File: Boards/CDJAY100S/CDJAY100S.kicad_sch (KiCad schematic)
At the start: 50 parts, among them SW1 RotaryEncoder_Switch, U1 HT1632C-52LQFP

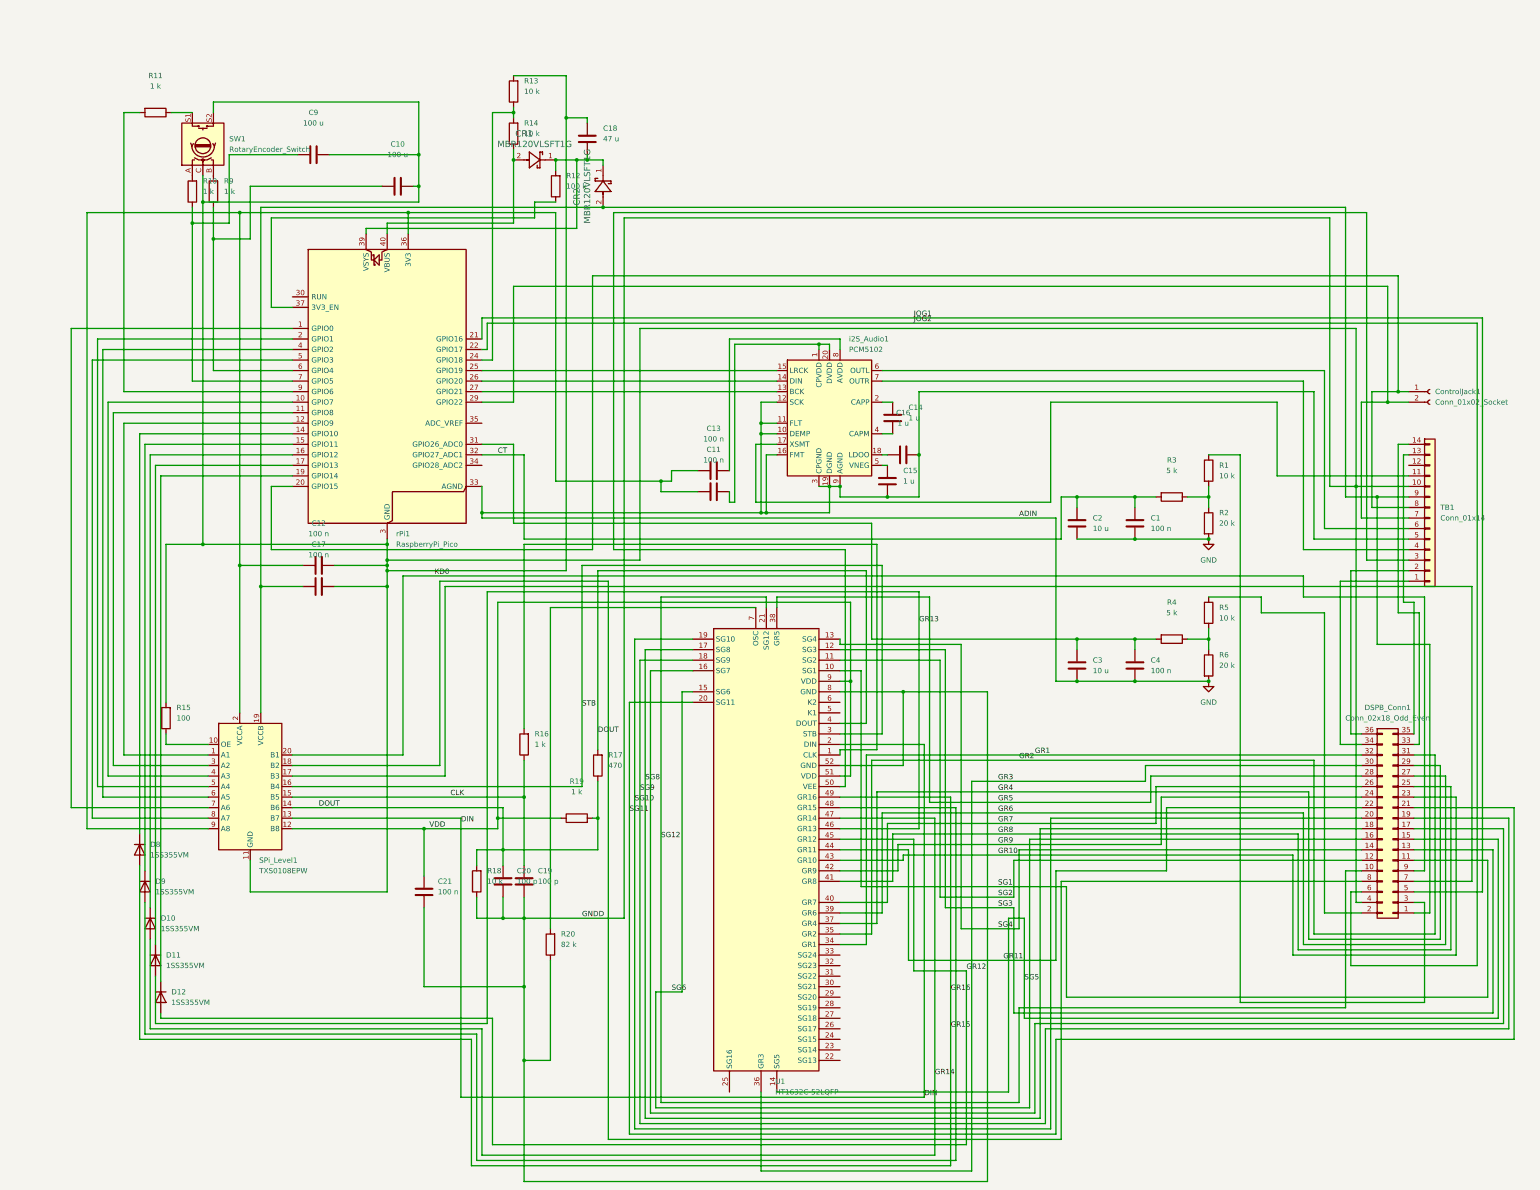
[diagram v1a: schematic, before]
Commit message: Revision 1.1 of the PCB and Schematics.
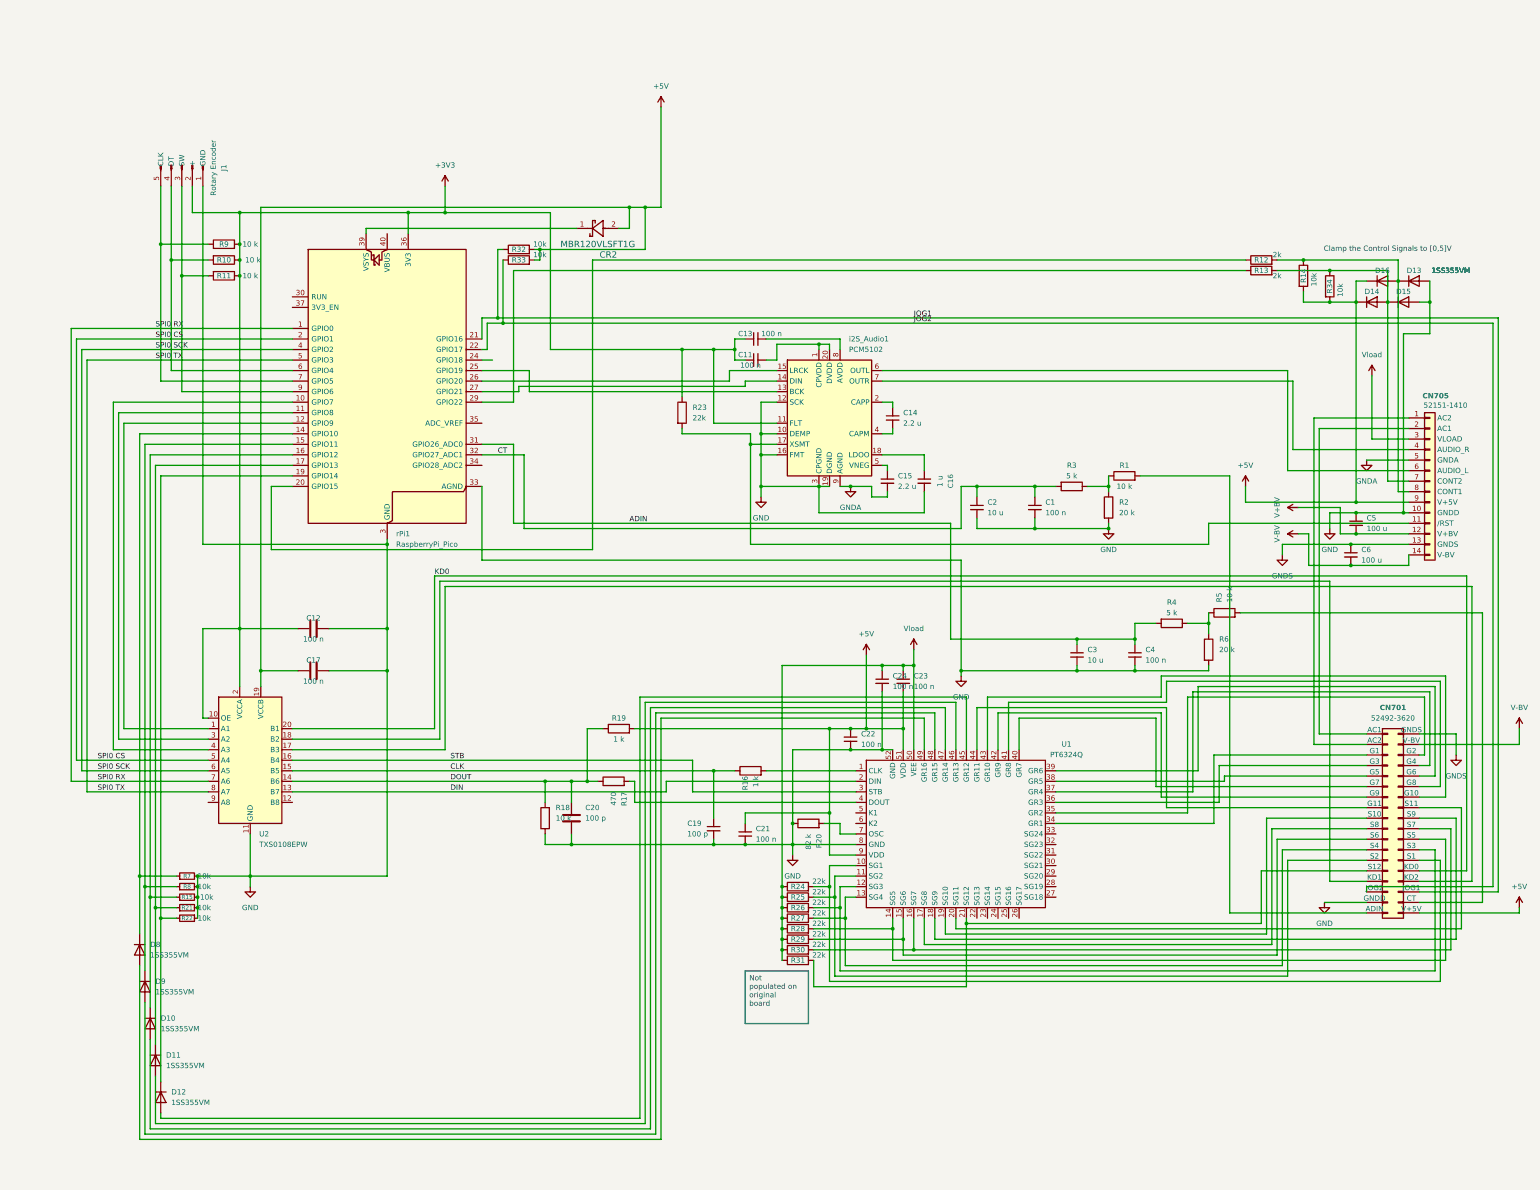
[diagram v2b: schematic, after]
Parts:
- removed C10, C9: 100 u, Capacitor_SMD:C_1206_3216Metric_Pad1.33x1.80mm_HandSolder, symbol Device:C
- removed C18: 47 u, Capacitor_SMD:C_1206_3216Metric_Pad1.33x1.80mm_HandSolder, symbol Device:C
- removed C19: 100 p, Capacitor_SMD:C_1206_3216Metric_Pad1.33x1.80mm_HandSolder, symbol Device:C
- removed C21: 100 n, Capacitor_SMD:C_1206_3216Metric_Pad1.33x1.80mm_HandSolder, symbol Device:C
- removed CR1: MBR120VLSFT1G, SDO_SOD-123FL_ONS, symbol 2026-07-07_11-12-20:MBR120VLSFT1G
- removed ControlJack1: Conn_01x02_Socket, Connector_Hirose:Hirose_DF13-02P-1.25DSA_1x02_P1.25mm_Vertical, symbol Connector:Conn_01x02_Socket
- removed DSPB_Conn1: Conn_02x18_Odd_Even, 52045-3645:ConnectorFPC&FFC_MOL52045-3645-36P, symbol Connector_Generic:Conn_02x18_Odd_Even
- removed R15: 100, Resistor_SMD:R_1206_3216Metric_Pad1.30x1.75mm_HandSolder, symbol Device:R
- removed SW1: RotaryEncoder_Switch, Connector_PinHeader_2.54mm:PinHeader_1x05_P2.54mm_Vertical, symbol Device:RotaryEncoder_Switch
- removed TB1: Conn_01x14, Connector_PinHeader_2.00mm:PinHeader_1x14_P2.00mm_Vertical, symbol Connector_Generic:Conn_01x14
- added C19: 100 p, Capacitor_SMD:C_1206_3216Metric_Pad1.33x1.80mm_HandSolder, symbol Device:C_Small
- added C21, C22, C23, C24: 100 n, Capacitor_SMD:C_1206_3216Metric_Pad1.33x1.80mm_HandSolder, symbol Device:C_Small
- added C5, C6: 100 u, Capacitor_SMD:C_1206_3216Metric_Pad1.33x1.80mm_HandSolder, symbol Device:C_Small
- added CN701: 52492-3620, 52045-3645:ConnectorFPC&FFC_MOL52045-3645-36P_1, symbol Connector_Generic:Conn_02x18_Odd_Even
- added CN705: 52151-1410, Connector_PinHeader_2.00mm:PinHeader_1x14_P2.00mm_Vertical, symbol Connector_Generic:Conn_01x14
- added D13, D14, D15, D16: 1SS355VM, Diode_SMD:Nexperia_CFP3_SOD-123W, symbol Diode:1SS355VM
- added J1: Rotary Encoder, Connector_PinHeader_2.54mm:PinHeader_1x05_P2.54mm_Vertical, symbol Connector:Conn_01x05_Pin
- added R15, R21, R22, R7, R8: 10k, Resistor_SMD:R_1206_3216Metric_Pad1.30x1.75mm_HandSolder, symbol Device:R_Small
- added R23, R24, R25, R26, R27, R28, R29, R30, R31: 22k, Resistor_SMD:R_1206_3216Metric_Pad1.30x1.75mm_HandSolder, symbol Device:R
- added R32, R33, R34: 10k, Resistor_SMD:R_1206_3216Metric_Pad1.30x1.75mm_HandSolder, symbol Device:R
- C1, C11, C13, C16, C2, C3, C4: symbol Device:C -> Device:C_Small
- C14, C15: value 1 u -> 2.2 u; symbol Device:C -> Device:C_Small
- CR2: footprint SDO_SOD-123FL_ONS -> Diode_SMD:Nexperia_CFP3_SOD-123W
- D10, D11, D12, D8, D9: footprint Diode_SMD:D_SOD-323F -> Diode_SMD:Nexperia_CFP3_SOD-123W
- R10, R11, R9: value 1 k -> 10 k
- R12: value 100 k -> 2k
- R13: value 10 k -> 2k
- R14: value 10 k -> 10k
- U1: value HT1632C-52LQFP -> PT6324Q; footprint Package_QFP:LQFP-52_14x14mm_P1mm -> Package_QFP:QFP-52_14x14mm_P1mm_1; symbol Driver_LED:HT1632C-52LQFP -> CDjay:PT6324
- renumbered SPi_Level1 to U2
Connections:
- net CLK: now also C19.1
- net DOUT: now also R19.1; no longer R17.2, R19.2, U1.4 (DOUT)
- net GND: now also C12.2, C17.2, C20.2, R18.1, R20.1, U1.52 (GND), U1.8 (GND), U2.11 (GND), rPi1.13 (GND), rPi1.18 (GND), rPi1.23 (GND), rPi1.28 (GND), rPi1.3 (GND), rPi1.38 (GND), rPi1.8 (GND), C19.2, C21.2, C22.2, C24.2, C5.1, CN701.4 (GNDD), CN705.10 (GNDD), D13.2 (A), D15.2 (A), J1.1 (GND), R15.2, R21.2, R22.1, R7.2, R8.2; no longer C15.2, i2S_Audio1.11 (FLT), i2S_Audio1.9 (AGND)
- net JOG1: now also CN701.5 (JOG1), R32.1
- net JOG2: now also CN701.6 (JOG2), R33.1
- net KD0: now also CN701.9 (KD0)
- net at R5.1: now also R4.1, R6.1
- net at D9.1 (K), rPi1.15 (GPIO11): now also R8.1
- net at R10.2: now also rPi1.6 (GPIO4), J1.4 (DT)
- net +3V3: now reaches R9.2
- net +3V3: now also C11.1, C12.1, C13.1, R10.1, R11.1, U2.10 (OE), U2.2 (VCCA), i2S_Audio1.11 (FLT), rPi1.36 (3V3), J1.2 (+), R23.1
- net at U2.17 (B3): now also CN701.7 (KD2)
- net at U2.18 (B2): now also CN701.8 (KD1)
- net +5V: now reaches C17.1, CR2.2, U2.19 (VCCB)
- net +5V: now also R14.2, R19.2, U1.51 (VDD), U1.9 (VDD), C21.1, C22.1, C23.2, CN701.1 (V+5V), CN705.9 (V+5V), D14.1 (K), D16.1 (K), R32.2, R33.2, R34.2
- net SPI0 CS: now reaches U2.5 (A4), rPi1.2 (GPIO1)
- net SPI0 SCK: now reaches U2.6 (A5), rPi1.4 (GPIO2)
- net SPI0 RX: now reaches U2.7 (A6), rPi1.1 (GPIO0)
- net SPI0 TX: now reaches U2.8 (A7), rPi1.5 (GPIO3)
- net at rPi1.7 (GPIO5): now also R9.1, J1.5 (CLK); no longer R10.1
- net at D11.1 (K), rPi1.17 (GPIO13): now also R21.1
- net at i2S_Audio1.17 (XSMT): now also CN705.11 (/RST), R23.2
- net Vload: now reaches U1.50 (VEE)
- net Vload: now also C23.1, C24.1, CN705.3 (VLOAD), R24.1, R25.1, R26.1, R27.1, R28.1, R29.1, R30.1, R31.1
- net at i2S_Audio1.7 (OUTR): now also CN705.4 (AUDIO_R)
- net at i2S_Audio1.6 (OUTL): now also CN705.6 (AUDIO_L)
- net at rPi1.29 (GPIO22): now also R13.1
- net at rPi1.20 (GPIO15): now also R12.1
- net ADIN: now reaches C3.1, C4.1, R4.2, rPi1.31 (GPIO26_ADC0)
- net at R1.1: now also R2.1, R3.1
- net at i2S_Audio1.13 (BCK): now also rPi1.25 (GPIO19); no longer rPi1.27 (GPIO21)
- net at i2S_Audio1.14 (DIN): now also rPi1.27 (GPIO21); no longer rPi1.26 (GPIO20)
- net at i2S_Audio1.15 (LRCK): now also rPi1.26 (GPIO20); no longer rPi1.25 (GPIO19)
- net at CR2.1, rPi1.39 (VSYS): no longer R12.2
- net at R14.1: now also R12.2, CN705.8 (CONT1), D13.1 (K), D16.2 (A); no longer rPi1.40 (VBUS)
- net at U1.16 (SG7): now also CN701.17 (S7), R30.2
- net at R11.2, rPi1.9 (GPIO6): now also J1.3 (SW)
- net at D8.1 (K), rPi1.14 (GPIO10): now also R7.1
- net at D10.1 (K), rPi1.16 (GPIO12): now also R15.1
- net at D12.1 (K), rPi1.19 (GPIO14): now also R22.2
- net at rPi1.37 (3V3_EN): no longer R12.1
- removed net GNDD: C12.2, C17.2, C20.2, R13.2, R18.1, R20.1, U1.52 (GND), U1.8 (GND), U2.11 (GND), rPi1.13 (GND), rPi1.18 (GND), rPi1.23 (GND), rPi1.28 (GND), rPi1.3 (GND), rPi1.38 (GND), rPi1.8 (GND)
- net GR1: no longer names the net of U1.34 (GR1)
- net GR1: now also CN701.32 (G1)
- net GR10: no longer names the net of U1.43 (GR10)
- net GR10: now also CN701.23 (G10)
- net GR11: no longer names the net of U1.44 (GR11)
- net GR11: now also CN701.22 (G11)
- net GR12: no longer names the net of D12.2 (A), U1.45 (GR12)
- net GR13: no longer names the net of D11.2 (A), U1.46 (GR13)
- net GR14: no longer names the net of D10.2 (A), U1.47 (GR14)
- net GR15: no longer names the net of D8.2 (A), U1.49 (GR16)
- net GR2: no longer names the net of U1.35 (GR2)
- net GR2: now also CN701.31 (G2)
- net GR3: no longer names the net of U1.36 (GR3)
- net GR3: now also CN701.30 (G3)
- net GR4: no longer names the net of U1.37 (GR4)
- net GR4: now also CN701.29 (G4)
- net GR5: no longer names the net of U1.38 (GR5)
- net GR5: now also CN701.28 (G5)
- net GR6: no longer names the net of U1.39 (GR6)
- net GR6: now also CN701.27 (G6)
- net GR7: no longer names the net of U1.40 (GR7)
- net GR7: now also CN701.26 (G7)
- net GR8: no longer names the net of U1.41 (GR8)
- net GR8: now also CN701.25 (G8)
- net GR9: no longer names the net of U1.42 (GR9)
- net GR9: now also CN701.24 (G9)
- net SG1: no longer names the net of U1.10 (SG1)
- net SG1: now also CN701.11 (S1), R24.2
- net SG10: no longer names the net of U1.19 (SG10)
- net SG10: now also CN701.20 (S10)
- net SG11: no longer names the net of U1.20 (SG11)
- net SG11: now also CN701.21 (S11)
- net SG12: no longer names the net of U1.21 (SG12)
- net SG12: now also CN701.10 (S12), R31.2
- net SG2: no longer names the net of U1.11 (SG2)
- net SG2: now also CN701.12 (S2), R25.2
- net SG3: no longer names the net of U1.12 (SG3)
- net SG3: now also CN701.13 (S3), R26.2
- net SG4: no longer names the net of U1.13 (SG4)
- net SG4: now also CN701.14 (S4), R27.2
- net SG5: no longer names the net of U1.14 (SG5)
- net SG5: now also CN701.15 (S5), R28.2
- net SG6: no longer names the net of U1.15 (SG6)
- net SG6: now also CN701.16 (S6), R29.2
- net SG8: no longer names the net of U1.17 (SG8)
- net SG8: now also CN701.18 (S8)
- net SG9: no longer names the net of U1.18 (SG9)
- net SG9: now also CN701.19 (S9)
- removed net VDD: R19.1, U1.51 (VDD), U1.9 (VDD), U2.12 (B8)
- new net: CN701.3 (CT), R5.2
- new net: CN701.2 (ADIN), R1.2
- new net: CN701.34 (AC2), CN705.1 (AC2)
- new net: CN701.36 (AC1), CN705.2 (AC1)
- new net: R17.2, U1.4 (DOUT)
- new net: CN705.7 (CONT2), D14.2 (A), D15.1 (K), R13.2, R34.1
- new net GNDA: C15.2, CN705.5 (GNDA), i2S_Audio1.9 (AGND)
- new net GNDS: C6.1, CN701.35 (GNDS), CN705.13 (GNDS)
- new net V+BV: C5.2, CN705.12 (V+BV)
- new net V-BV: C6.2, CN701.33 (V-BV), CN705.14 (V-BV)
- now unconnected: U2.9 (A8), rPi1.24 (GPIO18)
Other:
- note added: "Clamp the Control Signals to [0,5]V"
- company: (none) -> FH Aachen University of Applied Sciences
- title: (none) -> CDJay 100 Mainboard
- moved on the sheet: C1, C11, C12, C13, C16, C17, C2, C20, C3, C4, CR2, D10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
